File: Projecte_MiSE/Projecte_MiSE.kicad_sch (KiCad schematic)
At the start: 30 parts, among them J1 conn_DFrobot, U1 LMV324

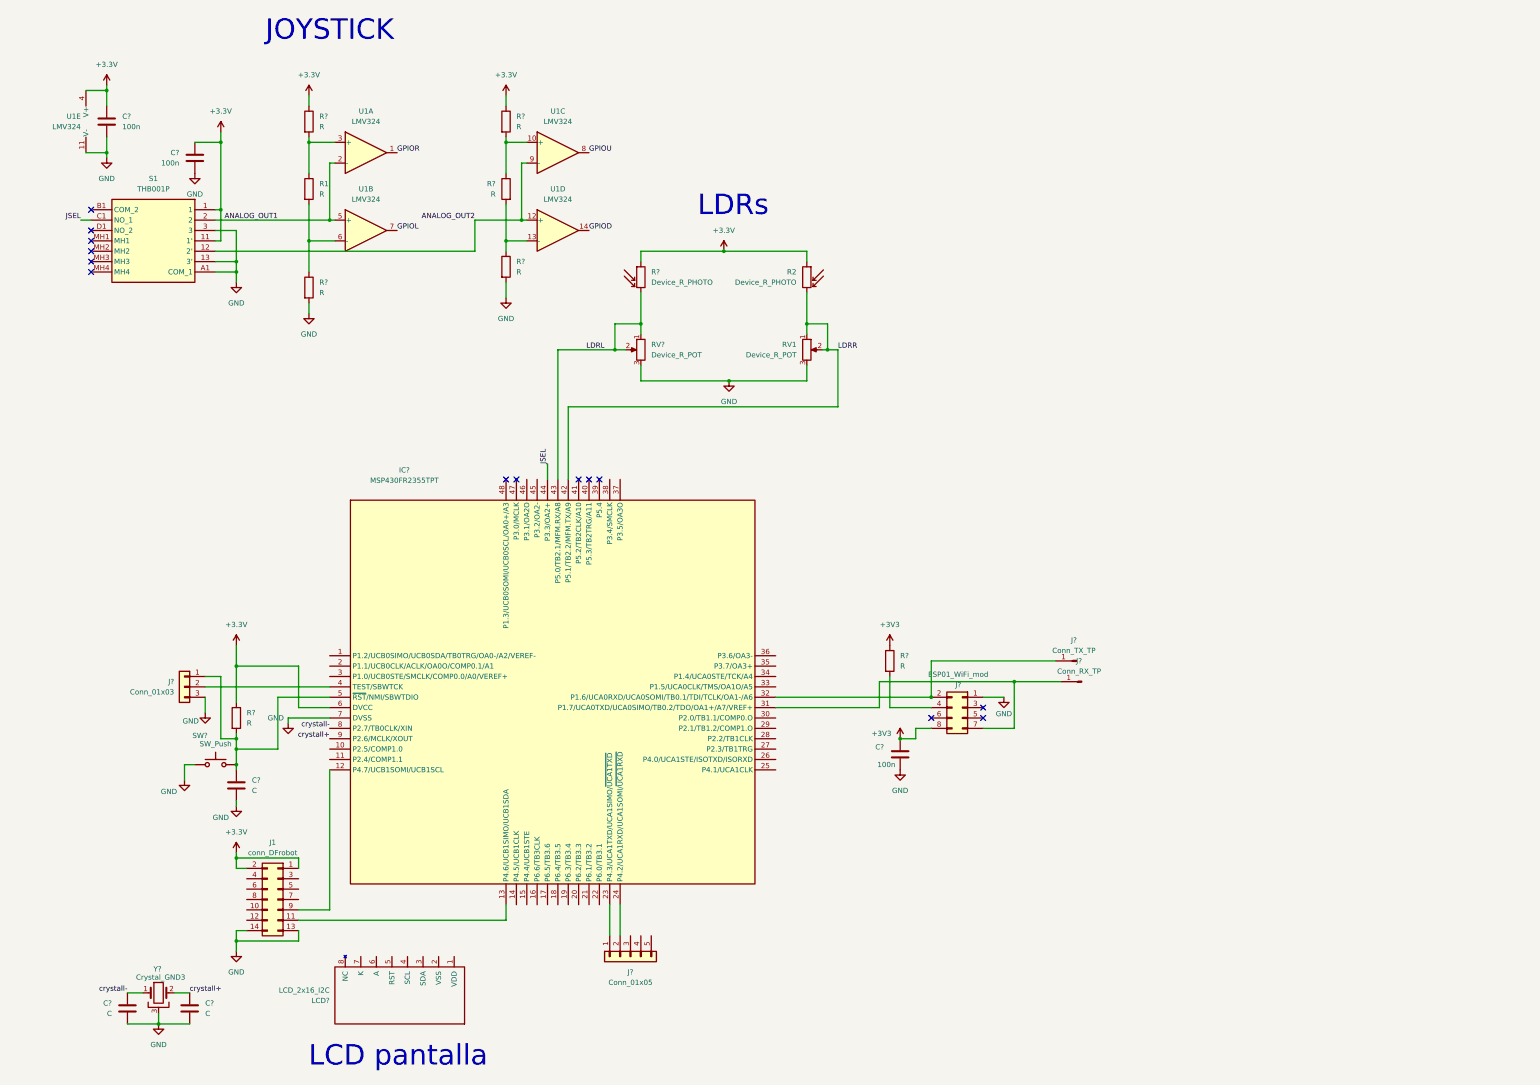
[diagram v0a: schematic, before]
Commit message: components add
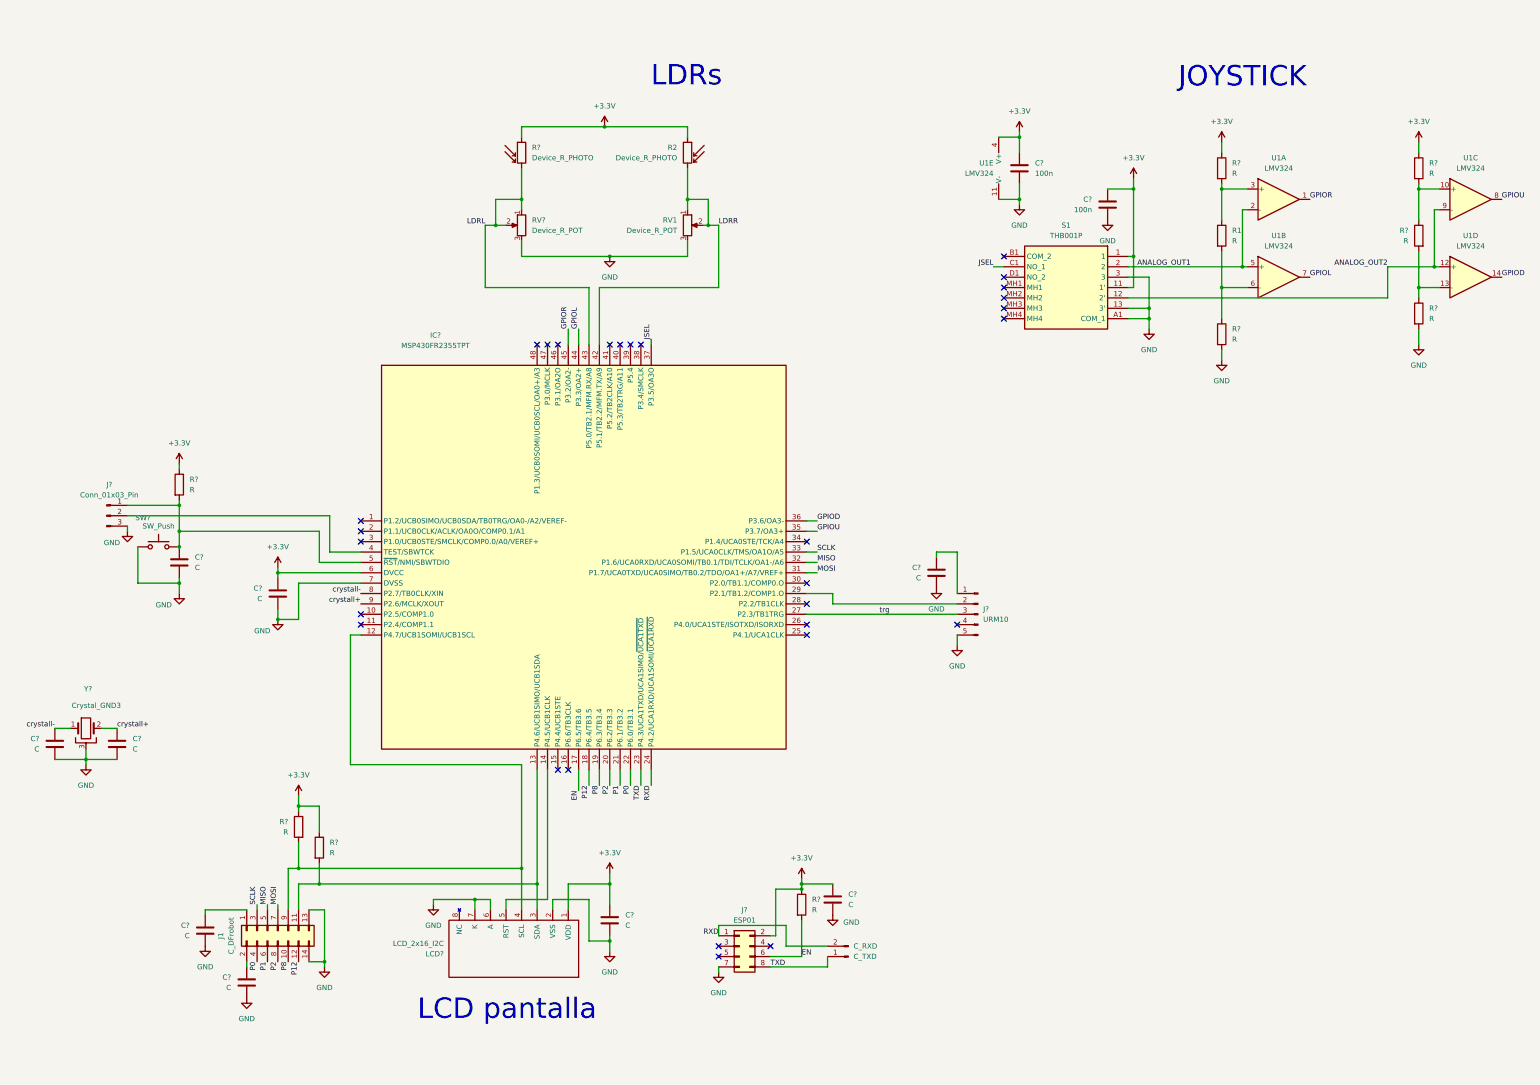
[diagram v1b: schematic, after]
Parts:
- removed C?: 100n, Capacitor_SMD:C_0805_2012Metric, symbol Device:C
- removed J?: ESP01_WiFi_mod, Connector_PinSocket_2.54mm:PinSocket_2x04_P2.54mm_Vertical, symbol Connector_Generic:Conn_02x04_Odd_Even
- removed J?: Conn_RX_TP, Connector_PinHeader_2.00mm:PinHeader_1x01_P2.00mm_Vertical, symbol Connector:Conn_01x01_Pin
- removed J?: Conn_TX_TP, Connector_PinHeader_2.00mm:PinHeader_1x01_P2.00mm_Vertical, symbol Connector:Conn_01x01_Pin
- removed J?: Conn_01x03, symbol Connector_Generic:Conn_01x03
- removed J?: Conn_01x05, symbol Connector_Generic:Conn_01x05
- removed R?: R, symbol Device:R
- added C? (x6): C, symbol Device:C
- added C_RXD: C_TXD, symbol Connector:Conn_01x02_Pin
- added J?: Conn_01x03_Pin, symbol Connector:Conn_01x03_Pin
- added J?: ESP01, symbol Connector_Generic:Conn_02x04_Odd_Even
- added J?: URM10, symbol Connector:Conn_01x05_Pin
- added R? (x3): R, symbol Device:R
- J1: value conn_DFrobot -> C_DFrobot
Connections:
- net +3.3V: now also LCD?.1 (VDD), C?.1, C?.1, C?.1, J?.2 (Pin_2), R?.1, R?.1, R?.1; no longer J1.1 (Pin_1), J1.2 (Pin_2)
- net GND: now also LCD?.2 (VSS), LCD?.6 (A), LCD?.7 (K), C?.2, C?.2, C?.2, C?.2, C?.2, C?.2, J?.3 (Pin_3), J?.5 (Pin_5), J?.7 (Pin_7)
- net GPIOD: now also IC?.36 (P3.6/OA3-)
- net GPIOL: now also IC?.44 (P3.3/OA2+)
- net GPIOR: now also IC?.45 (P3.2/OA2-)
- net GPIOU: now also IC?.35 (P3.7/OA3+)
- net JSEL: now also IC?.37 (P3.5/OA3O); no longer IC?.44 (P3.3/OA2+)
- net at IC?.12 (P4.7/UCB1SOMI/UCB1SCL), J1.9 (Pin_9): now also LCD?.4 (SCL), R?.2
- net at IC?.13 (P4.6/UCB1SIMO/UCB1SDA), J1.11 (Pin_11): now also LCD?.3 (SDA), R?.2
- net at IC?.14 (P4.5/UCB1CLK): now also LCD?.5 (RST)
- net EN: now reaches IC?.17 (P6.5/TB3.6)
- net EN: now also J?.6 (Pin_6), R?.2
- net P12: now reaches IC?.18 (P6.4/TB3.5)
- net P12: now also J1.12 (Pin_12)
- net P8: now reaches IC?.19 (P6.3/TB3.4)
- net P8: now also J1.10 (Pin_10)
- net P2: now reaches IC?.20 (P6.2/TB3.3)
- net P2: now also J1.8 (Pin_8)
- net P1: now reaches IC?.21 (P6.1/TB3.2)
- net P1: now also J1.6 (Pin_6)
- net P0: now reaches IC?.22 (P6.0/TB3.1)
- net P0: now also J1.4 (Pin_4)
- net TXD: now reaches IC?.23 (P4.3/UCA1TXD/UCA1SIMO/~{UCA1TXD})
- net TXD: now also C_RXD.1 (Pin_1), J?.8 (Pin_8)
- net RXD: now reaches IC?.24 (P4.2/UCA1RXD/UCA1SOMI/~{UCA1RXD})
- net RXD: now also C_RXD.2 (Pin_2), J?.1 (Pin_1)
- net trg: now reaches IC?.27 (P2.3/TB1TRG)
- net trg: now also J?.3 (Pin_3)
- net at IC?.29 (P2.1/TB1.2/COMP1.O): now also J?.2 (Pin_2)
- net MOSI: now reaches IC?.31 (P1.7/UCA0TXD/UCA0SIMO/TB0.2/TDO/OA1+/A7/VREF+)
- net MOSI: now also J1.7 (Pin_7)
- net MISO: now reaches IC?.32 (P1.6/UCA0RXD/UCA0SOMI/TB0.1/TDI/TCLK/OA1-/A6)
- net MISO: now also J1.5 (Pin_5)
- net SCLK: now reaches IC?.33 (P1.5/UCA0CLK/TMS/OA1O/A5)
- net SCLK: now also J1.3 (Pin_3)
- net at IC?.4 (TEST/SBWTCK): now also J?.2 (Pin_2)
- net at C?.1, IC?.5 (~{RST}/NMI/SBWTDIO), R?.2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: now also J?.1 (Pin_1)
- new net: C?.1, J1.1 (Pin_1)
- new net: C?.1, J?.1 (Pin_1)
- new net: C?.1, J1.2 (Pin_2)
- no-connect marks 14 -> 29
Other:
- moved on the sheet: C?, IC?, J1, LCD?, R1, R2, R?, RV1, RV?, S1, SW?, U1A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
